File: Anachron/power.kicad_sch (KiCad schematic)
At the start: 22 parts, among them J1 USB4520-03-0-A, Q1 AO3401A, SW1 Pad, U1 AP2112K-3.3TRG1, U2 MCP73831T-2ACI_OT

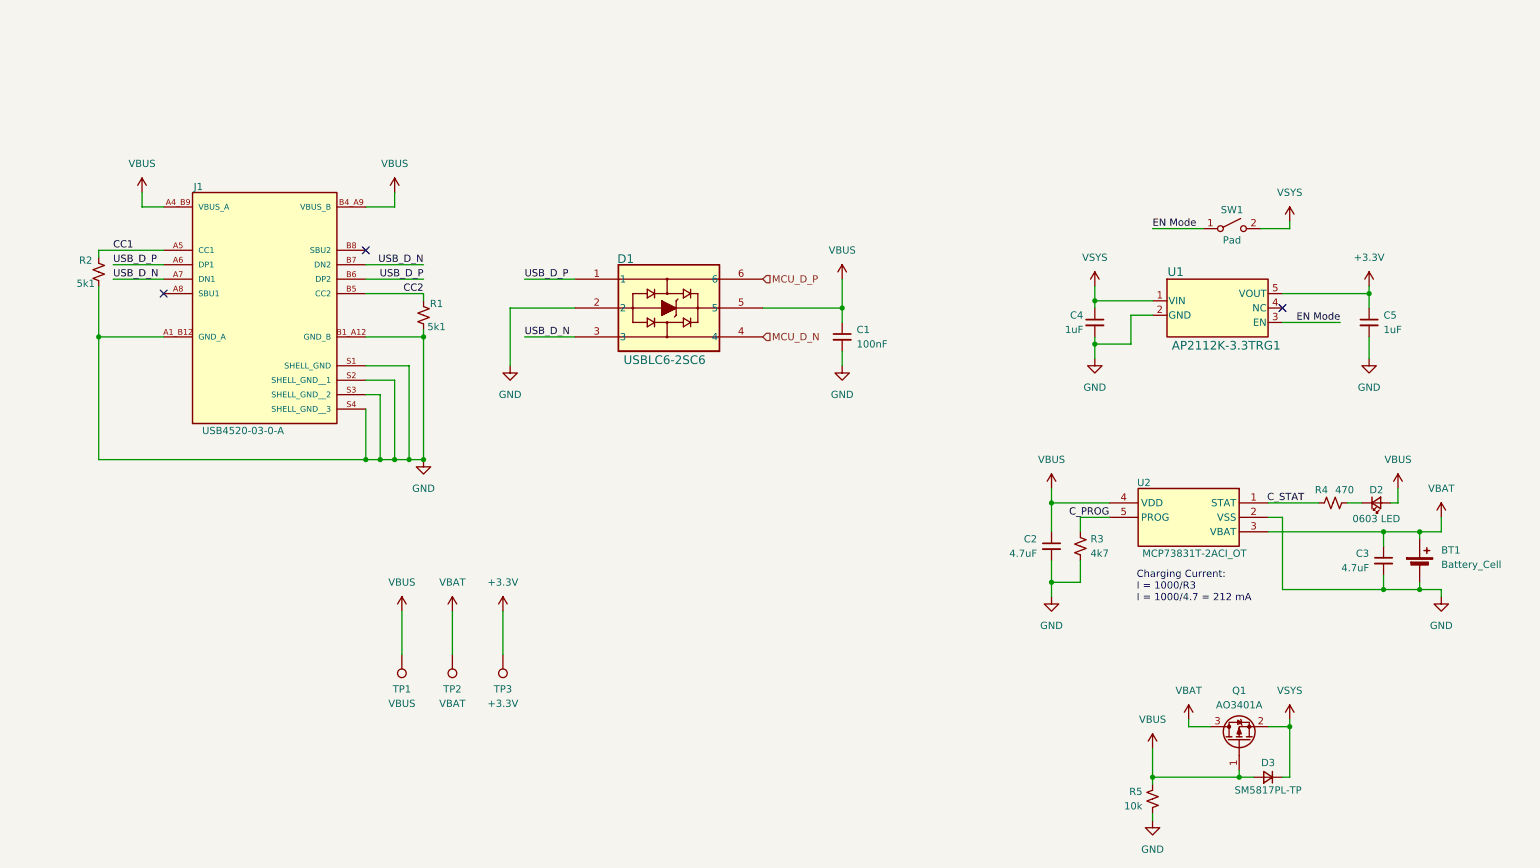
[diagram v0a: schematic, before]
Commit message: more changes!
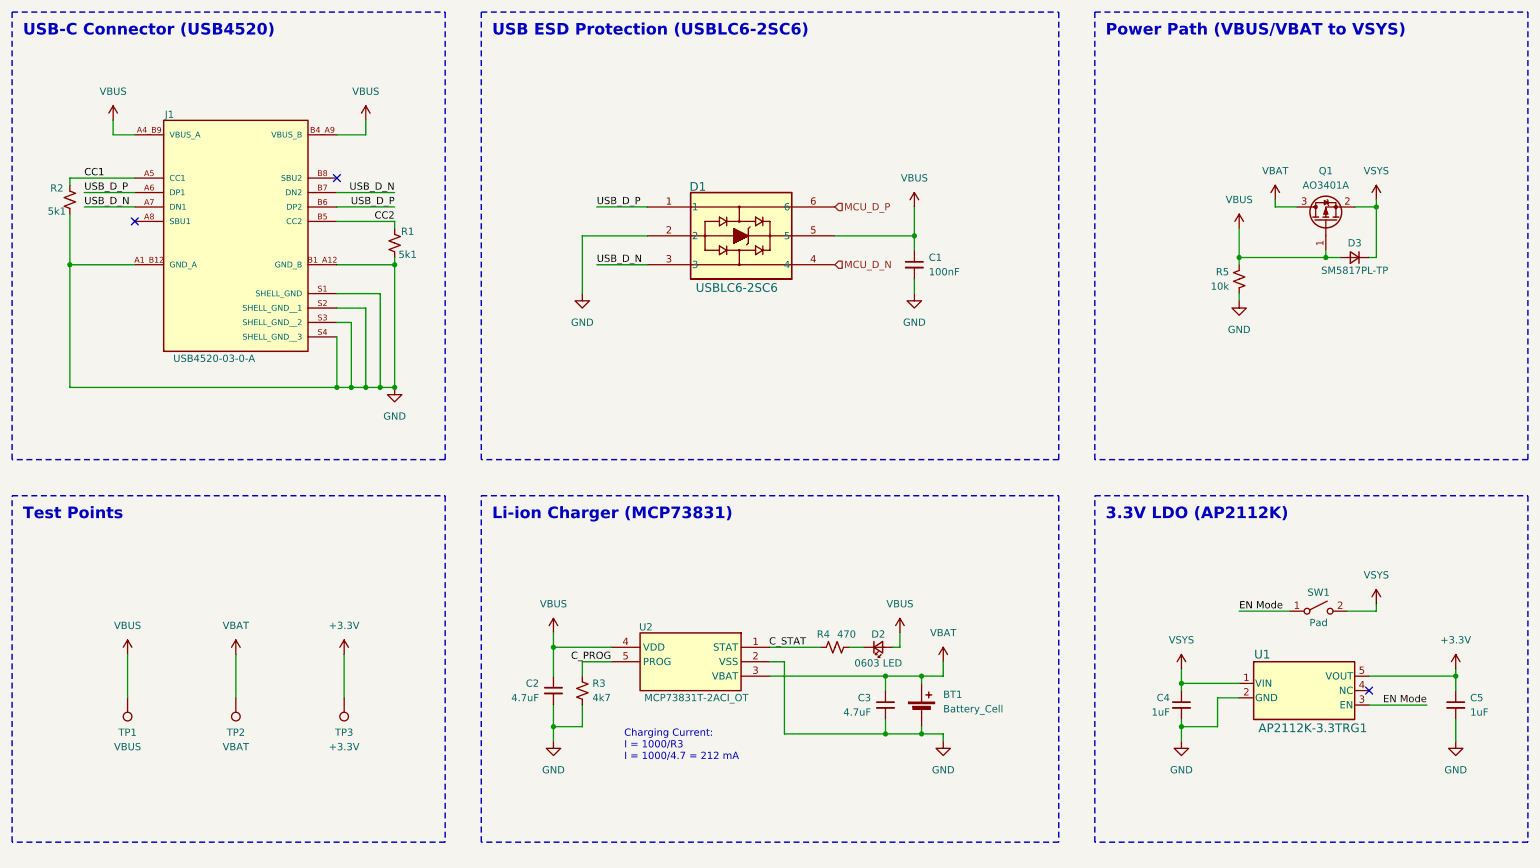
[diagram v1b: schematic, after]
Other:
- note added: "3.3V LDO (AP2112K)"
- note added: "Li-ion Charger (MCP73831)"
- note added: "Power Path (VBUS/VBAT to VSYS)"
- note added: "Test Points"
- note added: "USB ESD Protection (USBLC6-2SC6)"
- note added: "USB-C Connector (USB4520)"
- moved on the sheet: BT1, C1, C2, C3, C4, C5, D1, D2, D3, J1, Q1, R1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
